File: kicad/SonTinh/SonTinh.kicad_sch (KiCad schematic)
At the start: 9 parts, among them J8 791077010, U1 BME680, U2 TCA9517ADGK

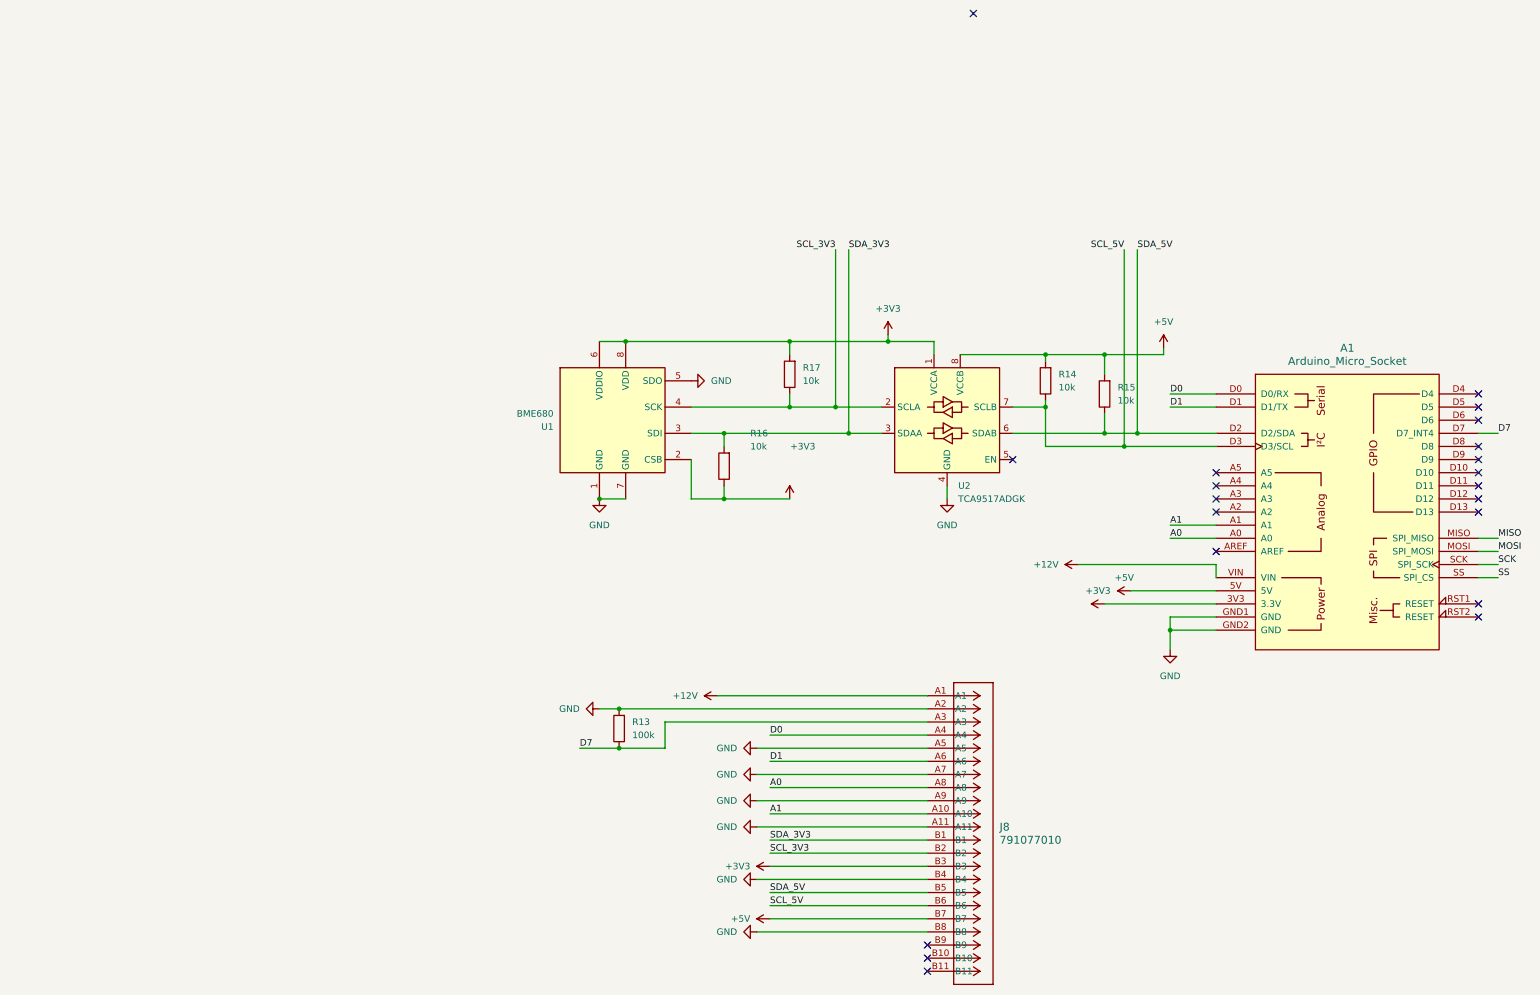
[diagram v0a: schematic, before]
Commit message: A Day in the Life
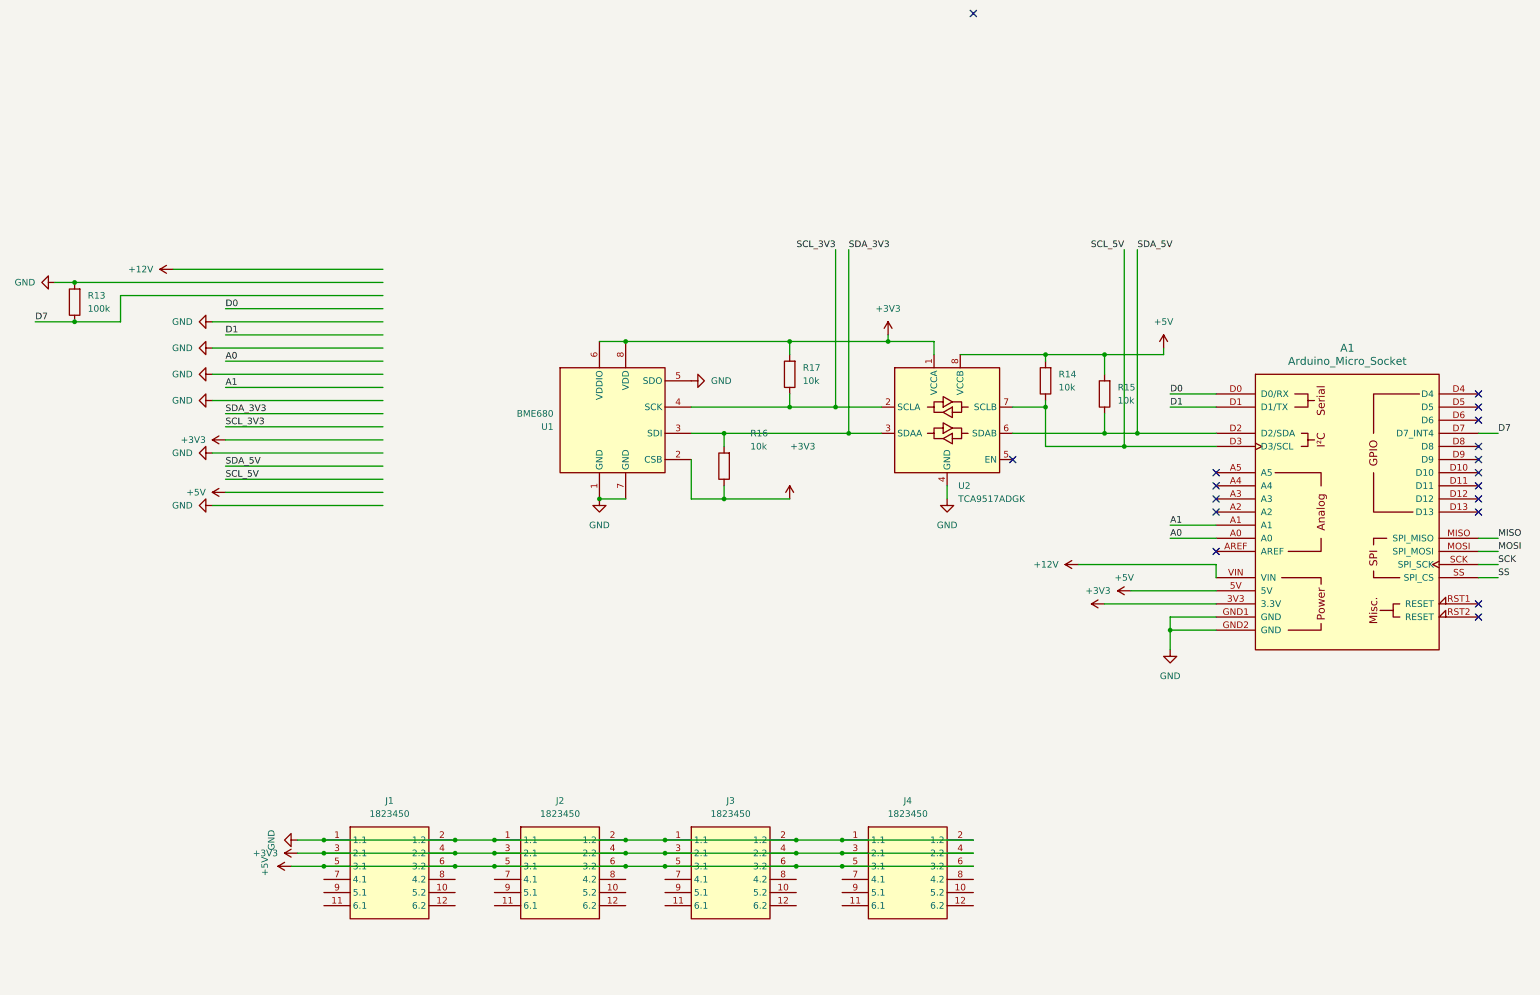
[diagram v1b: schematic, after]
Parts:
- removed J8: 791077010, footprints:CONN22_791077010_MOL, symbol Molex:791077010
- added J1, J2, J3, J4: 1823450, footprints:1823450, symbol PheonicContact:1823450
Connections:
- net +3V3: now also J1.3 (2.1), J1.4 (2.2), J2.3 (2.1), J2.4 (2.2), J3.3 (2.1), J3.4 (2.2), J4.3 (2.1), J4.4 (2.2)
- net +5V: now also J1.5 (3.1), J1.6 (3.2), J2.5 (3.1), J2.6 (3.2), J3.5 (3.1), J3.6 (3.2), J4.5 (3.1), J4.6 (3.2)
- net GND: now also J1.1 (1.1), J1.2 (1.2), J2.1 (1.1), J2.2 (1.2), J3.1 (1.1), J3.2 (1.2), J4.1 (1.1), J4.2 (1.2)
- no-connect marks 21 -> 18
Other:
- moved on the sheet: R13
